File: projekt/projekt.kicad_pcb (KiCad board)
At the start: 2 copper layers, 19 parts, among them J1 S8421-45R, SW1 SW_Push, U1 NE555P

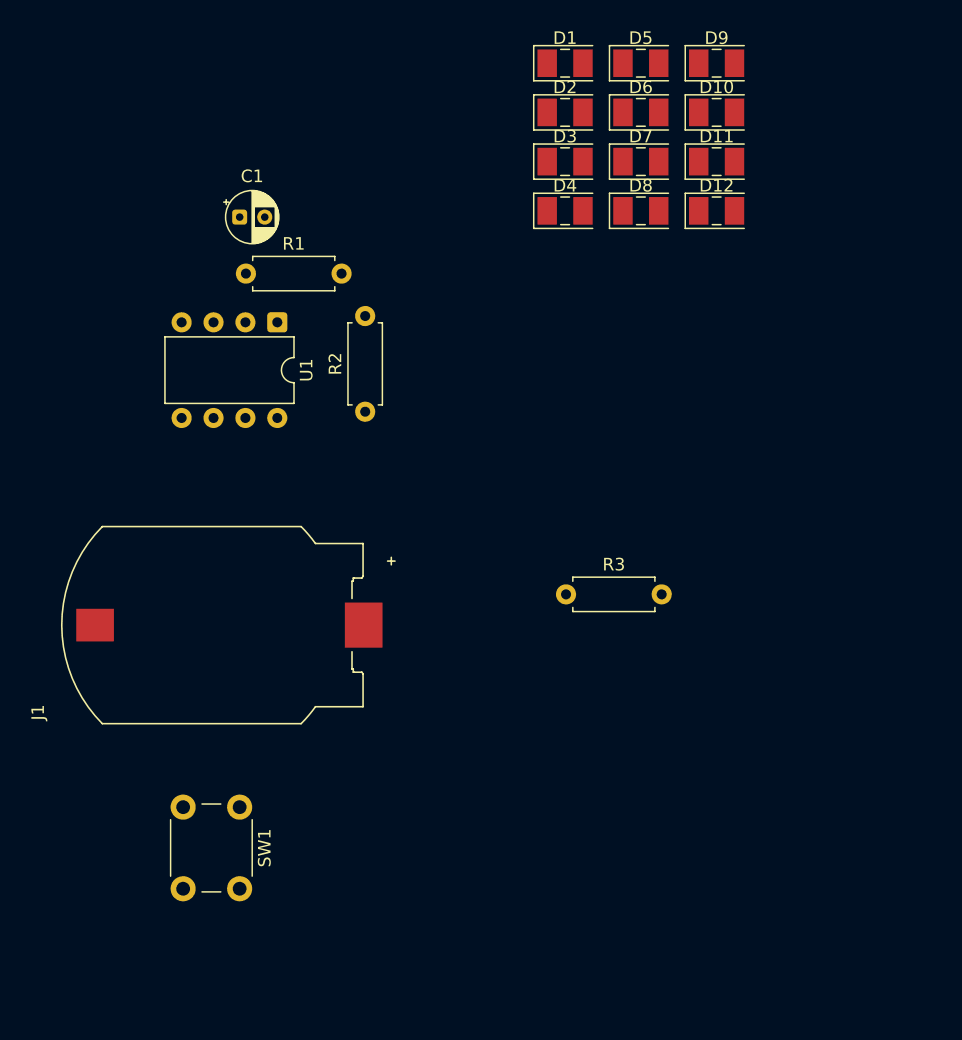
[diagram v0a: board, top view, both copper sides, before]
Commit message: wow! serduszko!
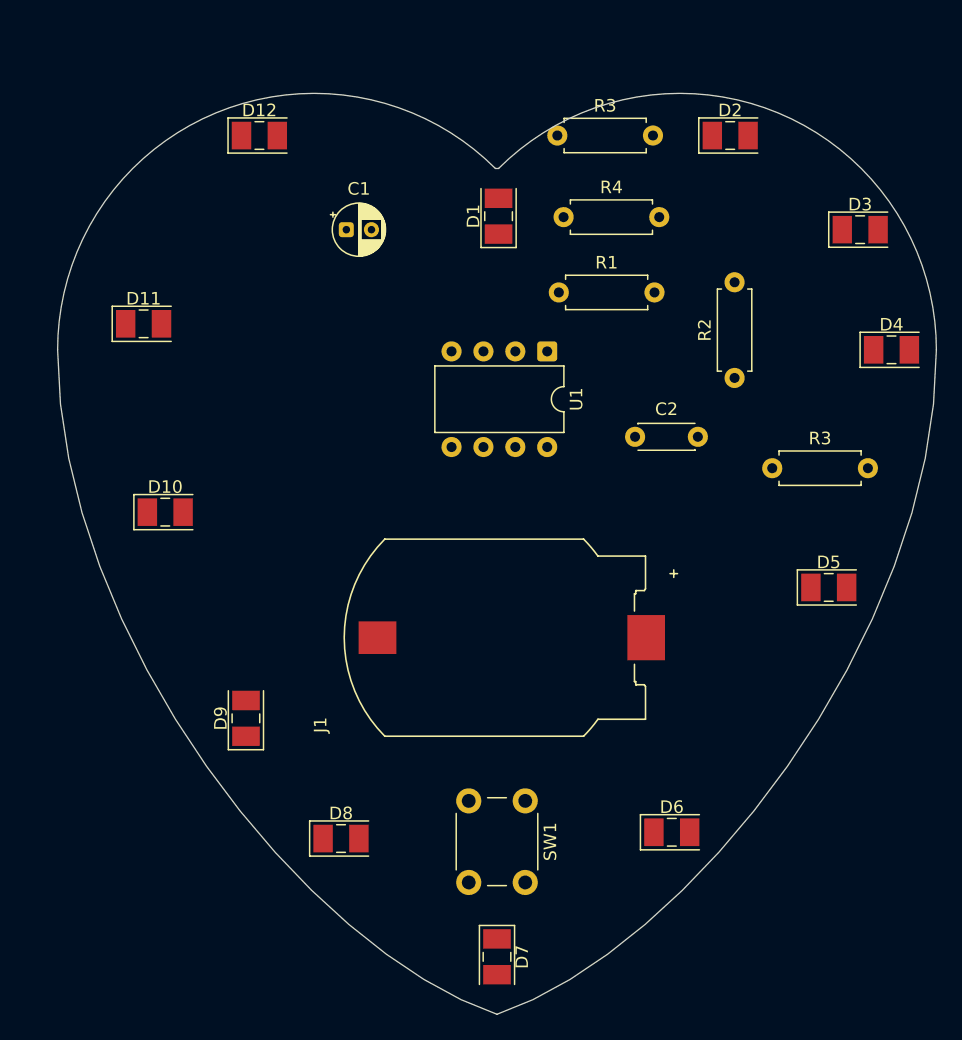
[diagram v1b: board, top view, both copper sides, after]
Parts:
- added C2: 10n, Capacitor_THT:C_Disc_D4.3mm_W1.9mm_P5.00mm, F.Cu at (181.0, 84.0)
- added R3: 100, Resistor_THT:R_Axial_DIN0207_L6.3mm_D2.5mm_P7.62mm_Horizontal, F.Cu at (174.8, 60.0)
- added R4: 100, Resistor_THT:R_Axial_DIN0207_L6.3mm_D2.5mm_P7.62mm_Horizontal, F.Cu at (175.3, 66.5)
- moved D7 64.4 mm to (170.0, 125.4), turned to -90 degrees
- moved D9 64.3 mm to (150.0, 106.4), turned to 90 degrees
- moved D6 57.4 mm to (183.9, 115.5)
- moved D8 55.4 mm to (157.6, 116.0)
- moved D10 54.2 mm to (143.6, 90.0)
- moved D11 47.4 mm to (141.8, 75.0)
- moved D5 44.4 mm to (196.4, 96.0)
- moved D12 36.9 mm to (151.1, 60.0)
- moved R2 29.5 mm to (188.9, 79.3)
- moved D4 28.3 mm to (201.4, 77.1)
- moved R1 25.0 mm to (174.9, 72.5)
- moved D3 24.1 mm to (198.9, 67.5)
- moved SW1 22.8 mm to (172.2, 113.0)
- moved J1 22.5 mm to (169.0, 100.0)
- moved U1 21.6 mm to (174.0, 77.2)
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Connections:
- D1 pad 1: GND -> Net-(D1-K)
- D1 pad 2: Net-(D1-A) -> /OUT
- D10 pad 2: VCC -> Net-(D10-A)
- D11 pad 1: GND -> Net-(D1-K)
- D11 pad 2: Net-(D1-A) -> /OUT
- D12 pad 1: Net-(D1-A) -> /OUT
- D12 pad 2: VCC -> Net-(D10-A)
- D2 pad 1: Net-(D1-A) -> /OUT
- D2 pad 2: VCC -> Net-(D10-A)
- D3 pad 1: GND -> Net-(D1-K)
- D4 pad 2: VCC -> Net-(D10-A)
- D5 pad 1: GND -> Net-(D1-K)
- D6 pad 2: VCC -> Net-(D10-A)
- D7 pad 1: GND -> Net-(D1-K)
- D8 pad 2: VCC -> Net-(D10-A)
- D9 pad 1: GND -> Net-(D1-K)
- U1 pad 5: GND -> Net-(U1-CV)
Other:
- board outline added: 70 x 73.4 mm
